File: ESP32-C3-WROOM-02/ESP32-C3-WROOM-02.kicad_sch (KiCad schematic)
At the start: 21 parts, among them J1 ESP32-C3-DEVKITC-02-J1, J2 ESP32-C3-DEVKITC-02-J2, J3 ESPProg-UART, J4 USB2.0_C, SW1 SW_Push, SW2 SW_Push, U1 AMS1117-3.3, U2 ESP32-C3-WROOM-02

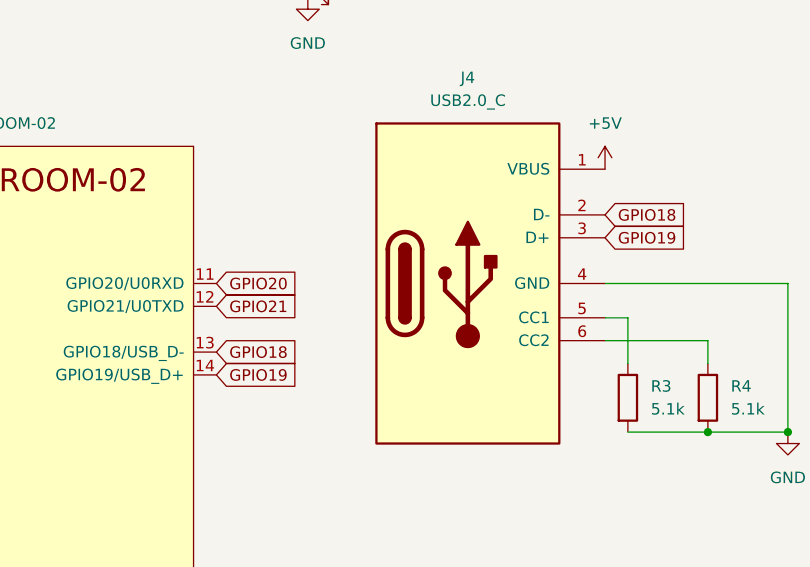
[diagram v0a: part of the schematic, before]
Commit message: ESP32C3Micro/v1.2.0
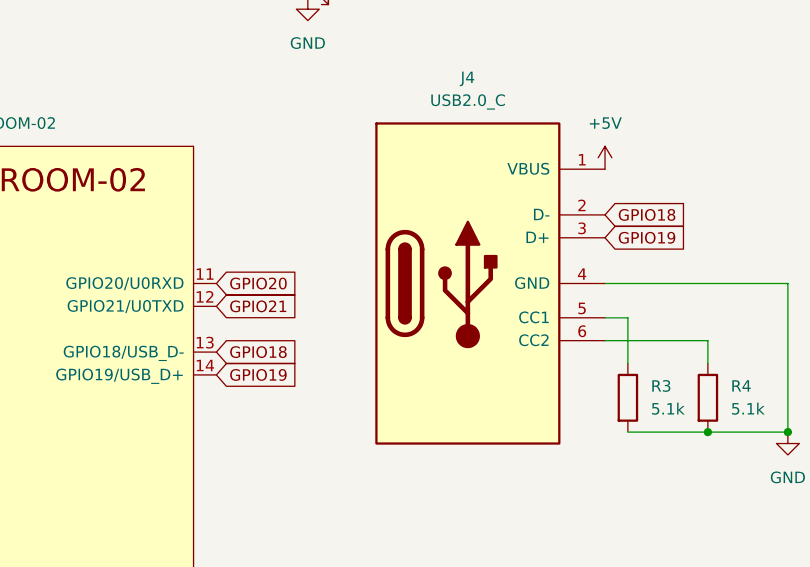
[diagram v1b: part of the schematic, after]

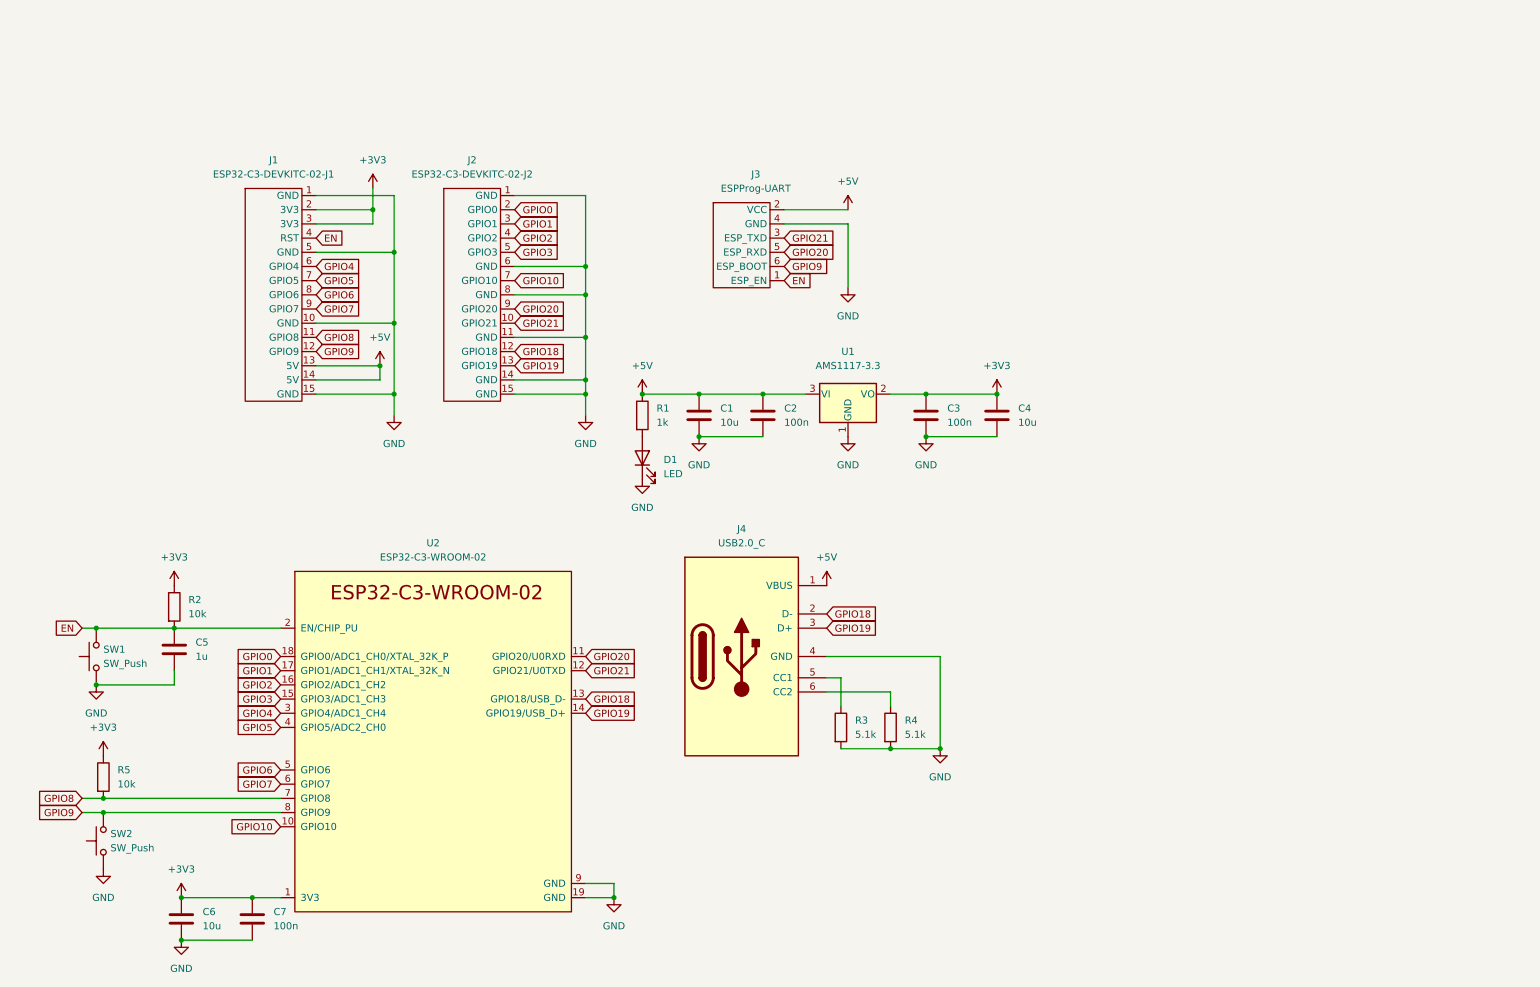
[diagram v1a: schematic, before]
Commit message: update
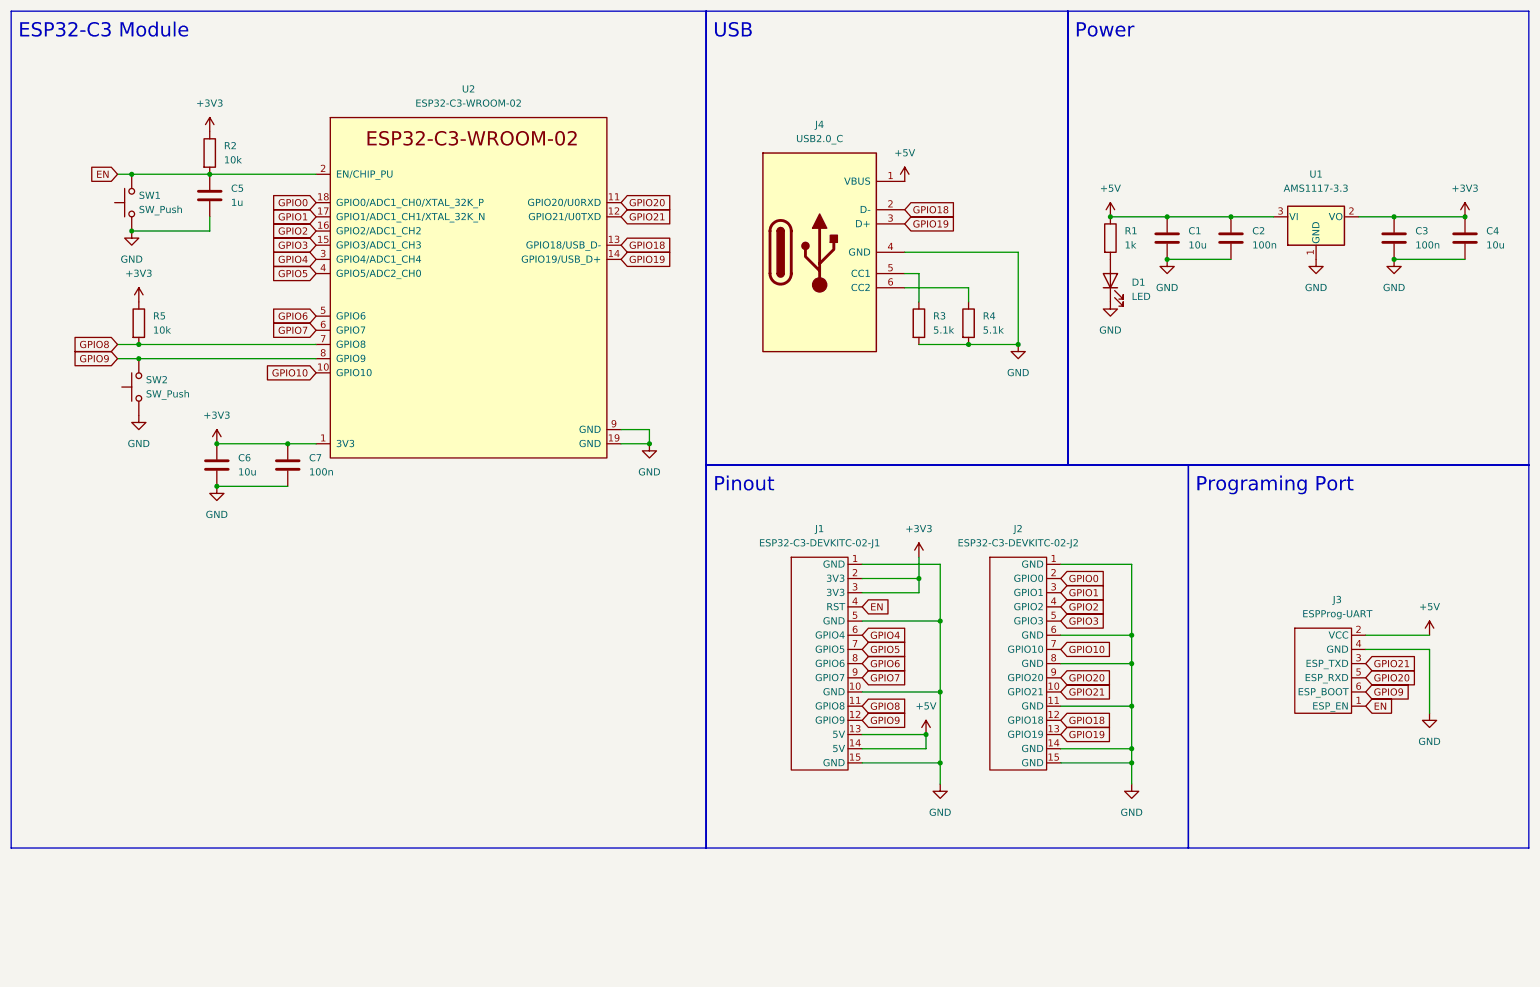
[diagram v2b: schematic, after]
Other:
- note added: "ESP32-C3 Module"
- note added: "Pinout"
- note added: "Power"
- note added: "Programing Port"
- note added: "USB"
- moved on the sheet: C1, C2, C3, C4, C5, C6, C7, D1, J1, J2, J3, J4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

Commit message: esp3s-c3-devboard/v1.2.0
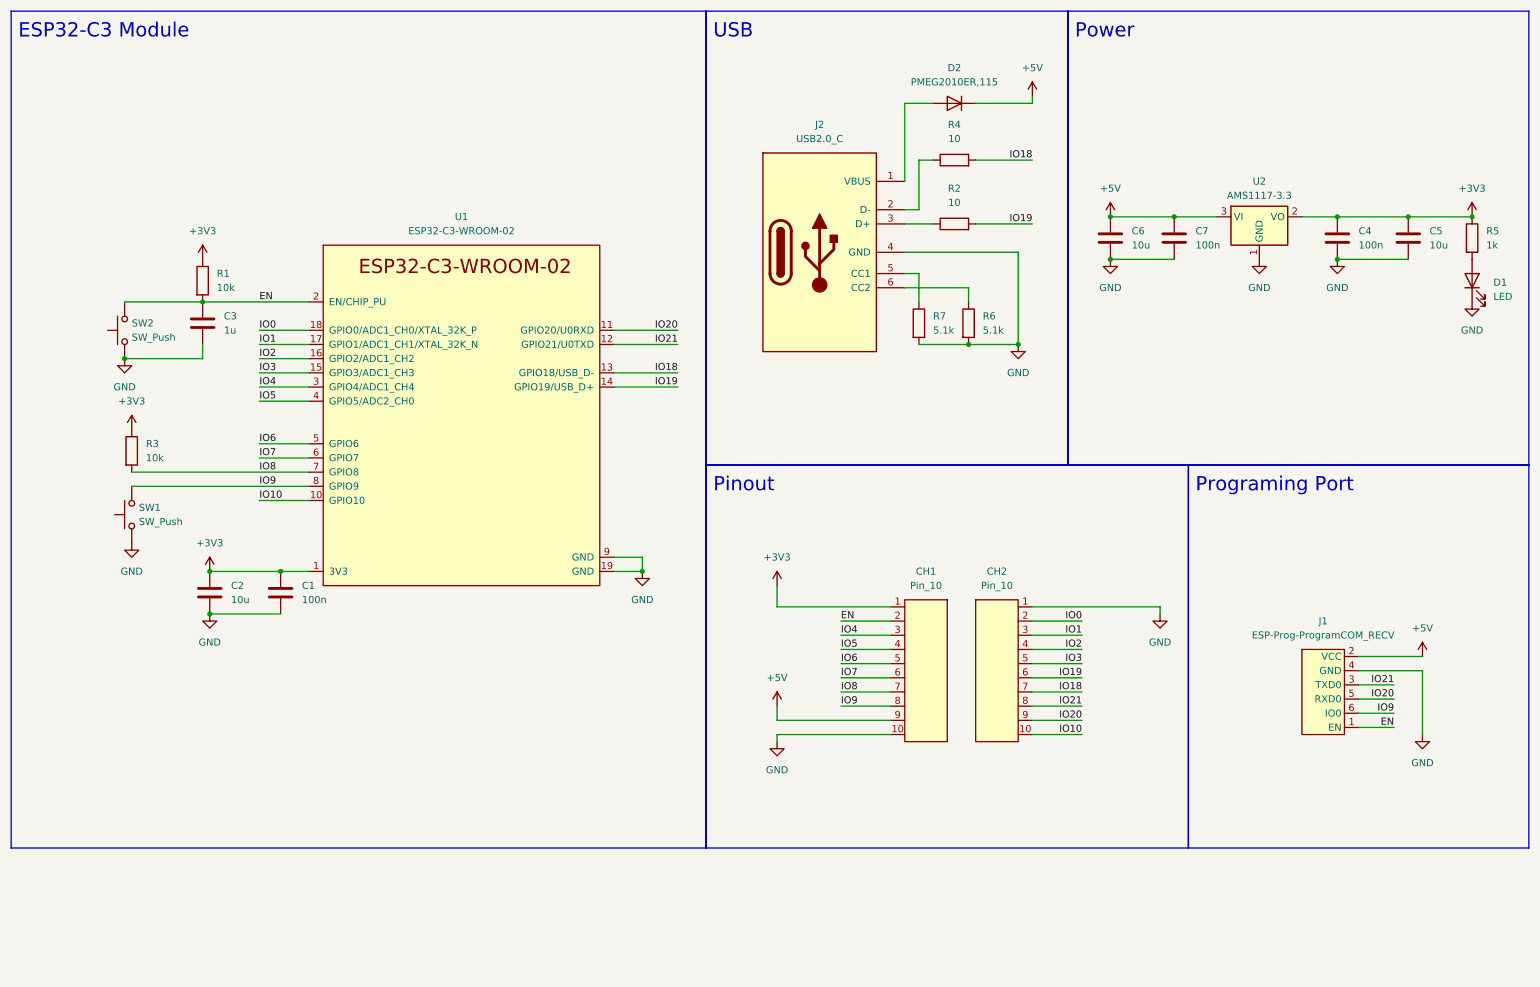
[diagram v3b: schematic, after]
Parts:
- removed J1: ESP32-C3-DEVKITC-02-J1, esp32-dev-board:ESP32-C3-DEVKITC-J1, symbol esp32-dev-board:ESP32-C3-DEVKITC-02-J1
- removed J2: ESP32-C3-DEVKITC-02-J2, esp32-dev-board:ESP32-C3-DEVKITC-J2, symbol esp32-dev-board:ESP32-C3-DEVKITC-02-J2
- removed J3: ESPProg-UART, esp32-dev-board:BoxPinHeader_2x03_P1.27mm_Vertical, symbol esp32-dev-board:ESPProg-UART
- added CH1, CH2: Pin_10, 74th:PinOut_Pin_10, symbol 74th_Interface:Pin_10
- added D2: PMEG2010ER,115, 74th:Package_SOD123W, symbol Device:D
- added J1: ESP-Prog-ProgramCOM_RECV, 74th:Connector_BoxPinHeader_2x03_P1.27mm, symbol 74th_Interface:ESP-Prog-ProgramCOM_RECV
- added R2, R4: 10, 74th:Register_0603_1608, symbol Device:R
- C1: renamed from C7; footprint esp32-dev-board:Capacitor_0805_2012 -> 74th:Capacitor_0603_1608
- C2: renamed from C6; footprint esp32-dev-board:Capacitor_0805_2012 -> 74th:Capacitor_0603_1608
- C3: renamed from C5; footprint esp32-dev-board:Capacitor_0805_2012 -> 74th:Capacitor_0603_1608
- C4: renamed from C3; footprint esp32-dev-board:Capacitor_0805_2012 -> 74th:Capacitor_0603_1608
- C5: renamed from C4; footprint esp32-dev-board:Capacitor_0805_2012 -> 74th:Capacitor_0603_1608
- C6: renamed from C1; footprint esp32-dev-board:Capacitor_0805_2012 -> 74th:Capacitor_0603_1608
- C7: renamed from C2; footprint esp32-dev-board:Capacitor_0805_2012 -> 74th:Capacitor_0603_1608
- D1: footprint LED_SMD:LED_0805_2012Metric_Pad1.15x1.40mm_HandSolder -> 74th:LED_0805_2012
- J2: renamed from J4; footprint esp32-dev-board:USB-C-12-Pin-MidMount-ali-v4 -> 74th:Connector_USB-C-Receptacle_SMT_12-Pin_Simple; symbol esp32-dev-board:USB2.0_C -> 74th_Interface:USB_TypeC-2.0_Receptacle
- R1: renamed from R2; footprint esp32-dev-board:Register_0805_2012 -> 74th:Register_0603_1608
- R3: renamed from R5; footprint esp32-dev-board:Register_0805_2012 -> 74th:Register_0603_1608
- R5: renamed from R1; footprint esp32-dev-board:Register_0805_2012 -> 74th:Register_0603_1608
- R6: renamed from R4; footprint esp32-dev-board:Register_0805_2012 -> 74th:Register_0603_1608
- R7: renamed from R3; footprint esp32-dev-board:Register_0805_2012 -> 74th:Register_0603_1608
- SW1: renamed from SW2; footprint esp32-dev-board:SKRPABE010 -> 74th:Switch_SKRPABE010
- SW2: renamed from SW1; footprint esp32-dev-board:SKRPABE010 -> 74th:Switch_SKRPABE010
- U1: renamed from U2; footprint esp32-dev-board:ESP32-C3-WROOM-02-handsolder -> PCM_Espressif:ESP32-C3-WROOM-02
- U2: renamed from U1; footprint Package_TO_SOT_SMD:SOT-223-3_TabPin2 -> 74th:Package_SOT-223-3; symbol Regulator_Linear:AMS1117-3.3 -> 74th_Passive:AMS1117-3.3_Regulator_SOT223
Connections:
- net +3V3: now also R5.1, CH1.1
- net +5V: now also CH1.9, D2.1 (K), J1.2 (VCC); no longer J2.1 (VBUS), R5.1
- net EN: now also CH1.2, J1.1 (EN)
- net GND: now also CH1.10, CH2.1, J1.4 (GND)
- net GPIO0 renamed IO0
- net IO0: now also CH2.2
- net GPIO1 renamed IO1
- net IO1: now also CH2.3
- net GPIO10 renamed IO10
- net IO10: now also CH2.10
- net GPIO18: no longer names the net of J2.2 (D-)
- net GPIO18: now also R4.1; no longer U1.13 (GPIO18/USB_D-)
- net GPIO19: no longer names the net of J2.3 (D+)
- net GPIO19: now also R2.1; no longer U1.14 (GPIO19/USB_D+)
- net GPIO2 renamed IO2
- net IO2: now also CH2.4
- net GPIO20 renamed IO20
- net IO20: now also CH2.9, J1.5 (RXD0)
- net GPIO21 renamed IO21
- net IO21: now also CH2.8, J1.3 (TXD0)
- net GPIO3 renamed IO3
- net IO3: now also CH2.5
- net GPIO4 renamed IO4
- net IO4: now also CH1.3
- net GPIO5 renamed IO5
- net IO5: now also CH1.4
- net GPIO6 renamed IO6
- net IO6: now also CH1.5
- net GPIO7 renamed IO7
- net IO7: now also CH1.6
- net GPIO8 renamed IO8
- net IO8: now also CH1.7
- net GPIO9 renamed IO9
- net IO9: now also CH1.8, J1.6 (IO0)
- new net: D2.2 (A), J2.1 (VBUS)
- new net IO18: CH2.7, R4.2, U1.13 (GPIO18/USB_D-)
- new net IO19: CH2.6, R2.2, U1.14 (GPIO19/USB_D+)
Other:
- moved on the sheet: C1, C2, C3, C4, C5, C6, C7, D1, R1, R3, R5, SW1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
